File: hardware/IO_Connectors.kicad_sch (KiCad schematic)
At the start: 31 parts, among them J29 RJ12_Shielded, J3 USB_B_Micro, U8 TJA1040

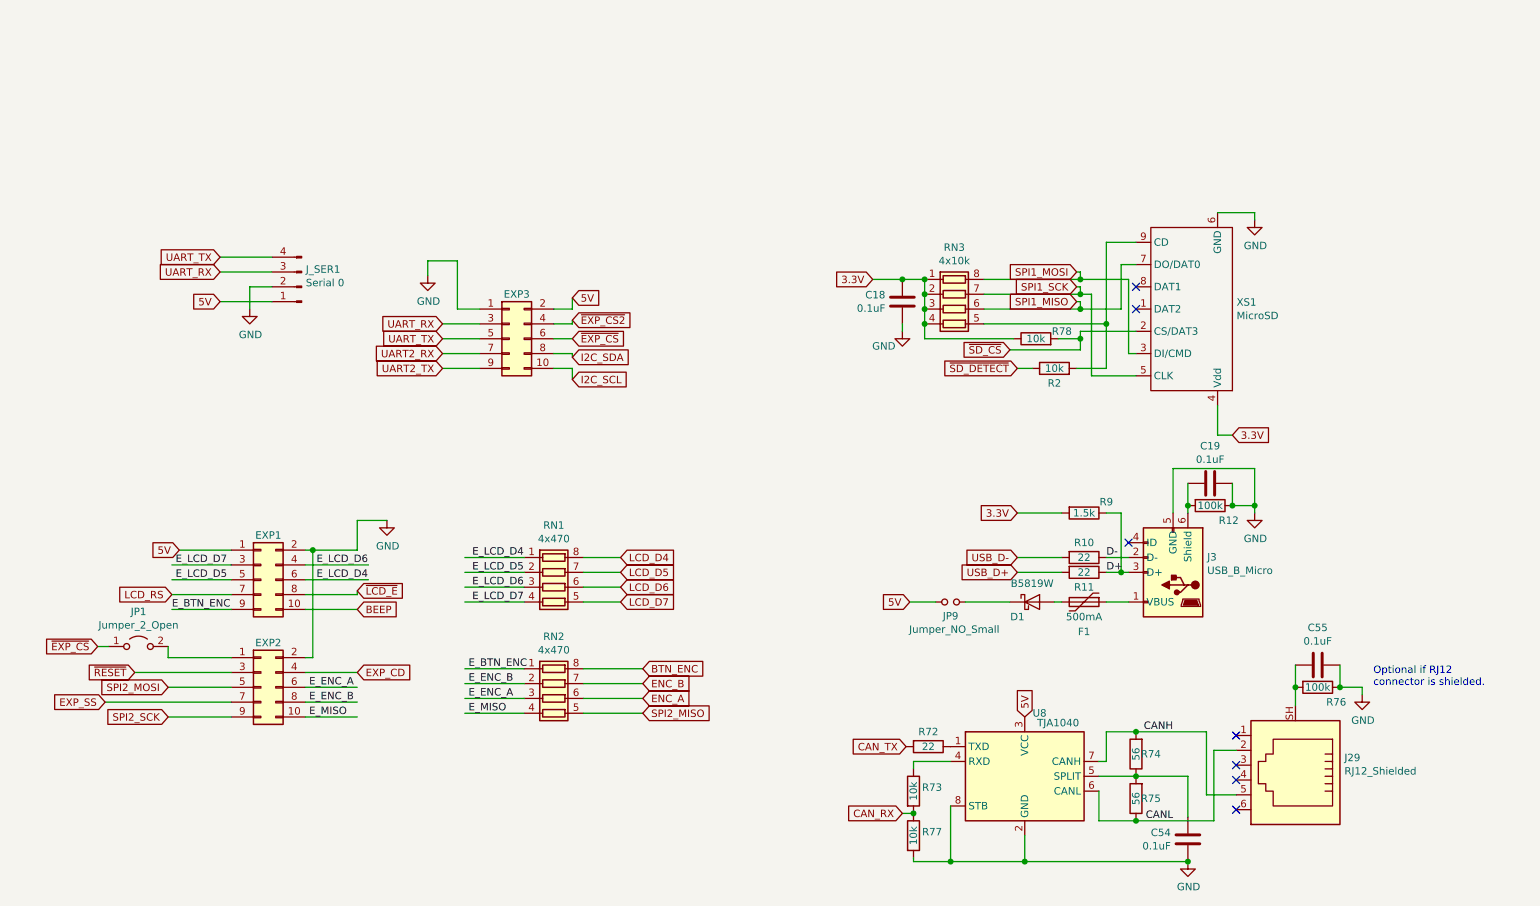
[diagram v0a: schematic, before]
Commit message: Intermediate checkin
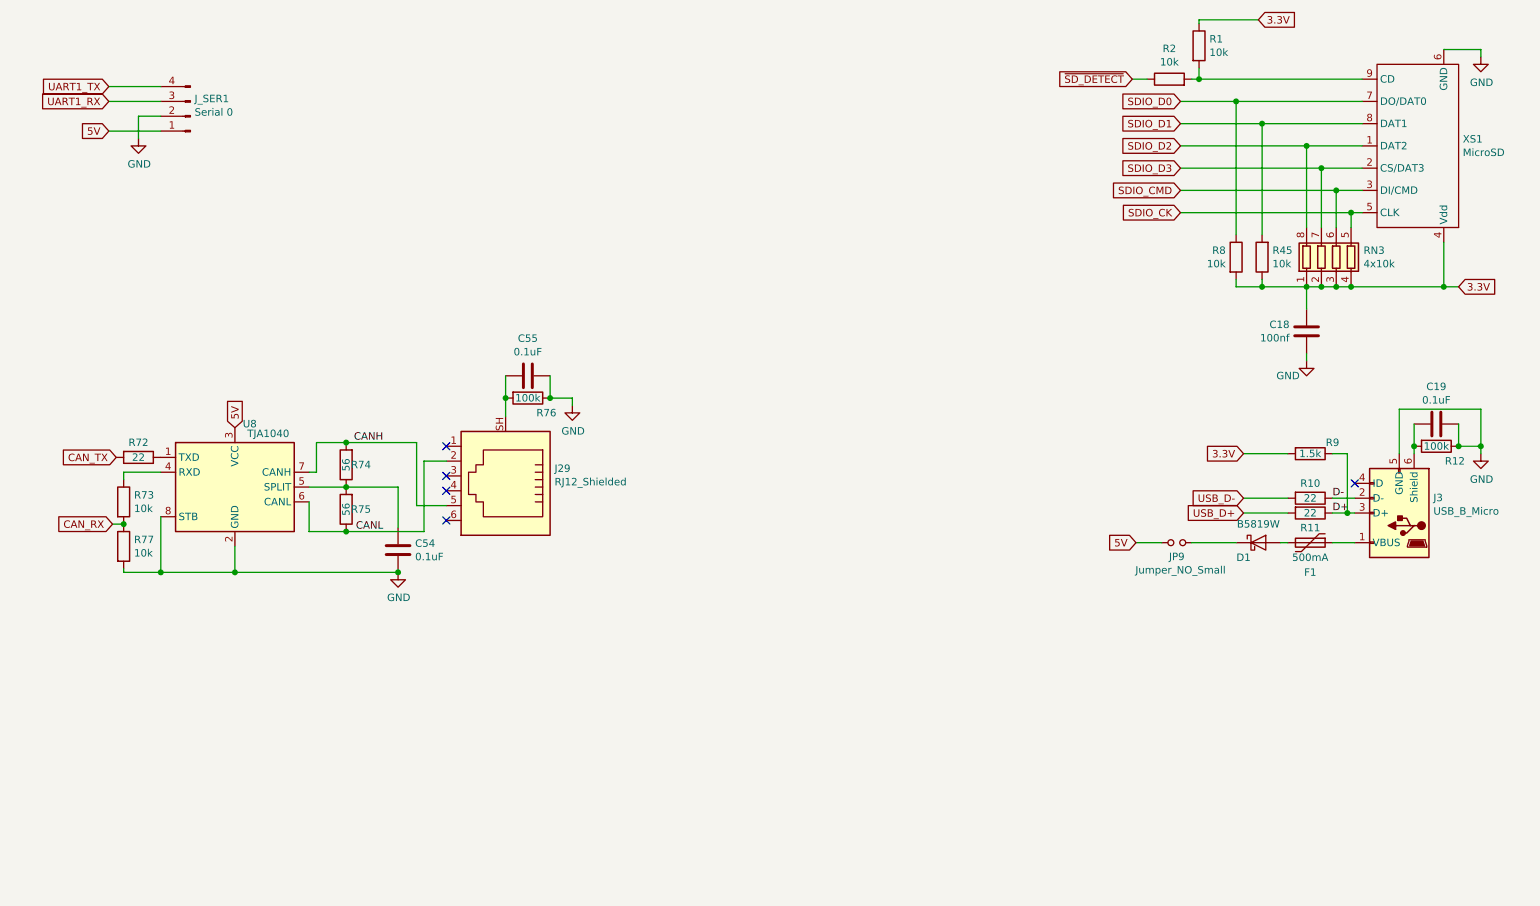
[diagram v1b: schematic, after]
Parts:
- removed EXP1, EXP2, EXP3: IDC 2x5, Connector_IDC:IDC-Header_2x05_P2.54mm_Vertical, symbol Connector_Generic:Conn_02x05_Odd_Even
- removed JP1: Jumper_2_Open, Connector_PinHeader_2.54mm:PinHeader_1x02_P2.54mm_Vertical, symbol Jumper:Jumper_2_Open
- removed R78: 10k, PrntrBoardV2:R_0603_1608Metric, symbol Device:R
- removed RN1, RN2: 4x470, Resistor_SMD:R_Array_Convex_4x0603, symbol Device:R_Pack04
- added R1, R45, R8: 10k, Resistor_SMD:R_0402_1005Metric, symbol Device:R
- C18: value 0.1uF -> 100nf; footprint PrntrBoardV2:C_0603_1608Metric -> Capacitor_SMD:C_0402_1005Metric; LCSC Part # C14663 -> C1525; Part # CC0603KRX7R9BB104 -> CL05B104KO5NNNC
- C19, C54: footprint PrntrBoardV2:C_0603_1608Metric -> Capacitor_SMD:C_0402_1005Metric; LCSC Part # C14663 -> C1525; Part # CC0603KRX7R9BB104 -> CL05B104KO5NNNC
- C55: footprint PrntrBoardV2:C_0603_1608Metric -> Capacitor_SMD:C_0402_1005Metric; LCSC Part # C14663 -> C1525; Part # CC0603KRX7R9BB104 -> CL05B104KO5NNNC; now in the parts list
- J29: footprint Connector_RJ:RJ12_Amphenol_54601 -> PrntrBoardV2:Wurth_615006143421
- R10, R11, R72: footprint PrntrBoardV2:R_0603_1608Metric -> Resistor_SMD:R_0402_1005Metric; LCSC Part # C23345 -> C25092; Part # 0603WAF220JT5E -> 0402WGF220JTCE
- R12: footprint PrntrBoardV2:R_0603_1608Metric -> Resistor_SMD:R_0402_1005Metric; LCSC Part # C25803 -> C25741; Part # 0603WAF1003T5E -> 0402WGF1003TCE
- R2, R73, R77: footprint PrntrBoardV2:R_0603_1608Metric -> Resistor_SMD:R_0402_1005Metric; LCSC Part # C25804 -> C25744; Part # 0603WAF1002T5E -> 0402WGF1002TCE
- R74, R75: footprint PrntrBoardV2:R_0603_1608Metric -> Resistor_SMD:R_0603_1608Metric
- R76: footprint PrntrBoardV2:R_0603_1608Metric -> Resistor_SMD:R_0402_1005Metric; LCSC Part # C25803 -> C25741; Part # 0603WAF1003T5E -> 0402WGF1003TCE; now in the parts list
- R9: footprint PrntrBoardV2:R_0603_1608Metric -> Resistor_SMD:R_0402_1005Metric; LCSC Part # C22843 -> C25867; Part # 0603WAF1501T5E -> 0402WGF1501TCE
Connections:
- net 3.3V: now also R1.1, R45.1, R8.2
- net SDIO_D2: now reaches XS1.1 (DAT2)
- net SDIO_D2: now also RN3.8 (R1.2)
- net SDIO_D1: now reaches XS1.8 (DAT1)
- net SDIO_D1: now also R45.2
- net at R2.2, XS1.9 (CD): now also R1.2; no longer RN3.5 (R4.2)
- net SPI1_MISO renamed SDIO_CMD
- net SDIO_CMD: now also XS1.3 (DI/CMD); no longer XS1.7 (DO/DAT0)
- removed net SPI1_MOSI: RN3.8 (R1.2), XS1.3 (DI/CMD)
- net SPI1_SCK renamed SDIO_CK
- net SDIO_CK: now also RN3.5 (R4.2); no longer RN3.7 (R2.2)
- net UART_RX renamed UART1_RX
- net UART_TX renamed UART1_TX
- net ~SD_CS renamed SDIO_D3
- net SDIO_D3: now also RN3.7 (R2.2)
- new net SDIO_D0: R8.1, XS1.7 (DO/DAT0)
- no-connect marks 7 -> 5
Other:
- note removed: "Optional if RJ12 connector is shielded."
- moved on the sheet: C18, C19, C54, C55, D1, F1, J29, J3, JP9, J_SER1, R10, R11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
